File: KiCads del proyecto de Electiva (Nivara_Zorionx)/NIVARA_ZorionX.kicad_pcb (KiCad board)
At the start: 4 copper layers, 109.1 x 87.7 mm, 77 parts, among them J1 Screw_Terminal_01x03, J10 Screw_Terminal_01x03, J11 Screw_Terminal_01x03, J2 Screw_Terminal_01x03, J3 Screw_Terminal_01x04, J4 Screw_Terminal_01x03, J5 Screw_Terminal_01x02, J6 Screw_Terminal_01x02, J7 Screw_Terminal_01x03, J8 Screw_Terminal_01x04, J9 Screw_Terminal_01x06, K1 G2RL-1, K2 G2RL-1, U1 ESP32-S3-WROOM-1, U11 LTV-357TB, U12 LTV-357TB, U2 AP63200WU, U4 LTV-357TB, U5 LTV-357TB, U8 LTV-357TB, U9 LTV-357TB

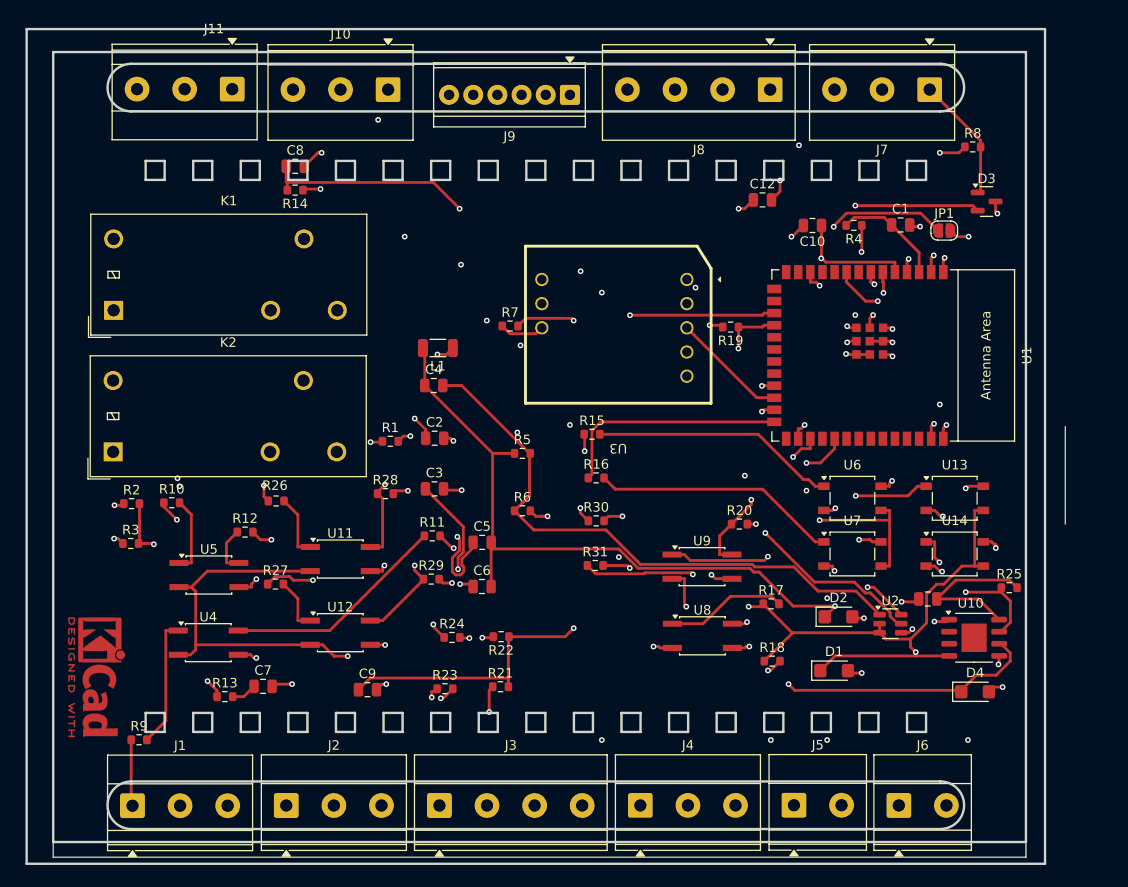
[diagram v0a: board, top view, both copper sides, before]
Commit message: Papadio Dame Fuerza
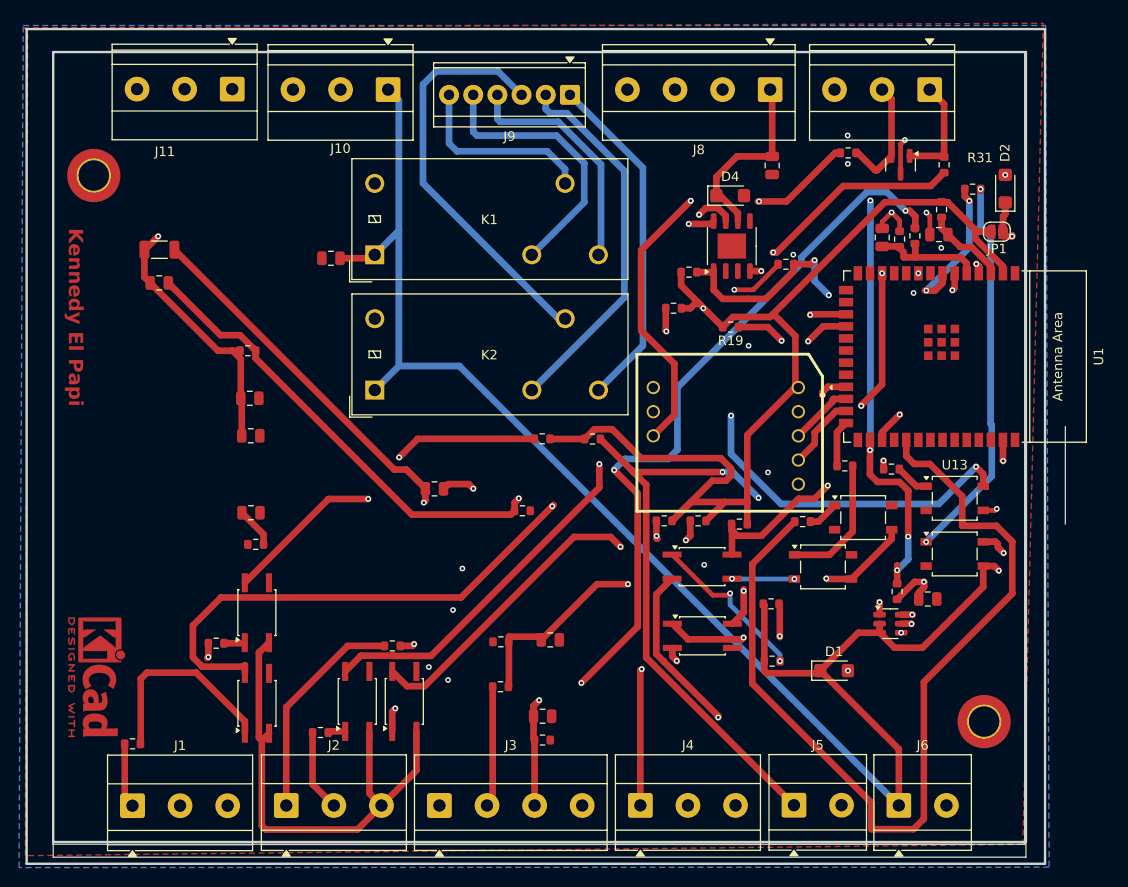
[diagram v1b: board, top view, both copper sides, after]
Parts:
- added REF**: MountingHole_3.2mm_M3_DIN965_Pad_TopOnly, MountingHole:MountingHole_3.2mm_M3_DIN965_Pad_TopOnly, F.Cu at (36.2, 41.4)
- added REF**: MountingHole_3.2mm_M3_DIN965_Pad_TopOnly, MountingHole:MountingHole_3.2mm_M3_DIN965_Pad_TopOnly, F.Cu at (129.7, 98.8)
- moved R3 74.8 mm to (108.9, 50.7)
- moved R23 68.6 mm to (122.5, 47.7), turned to -90 degrees
- moved R2 63.4 mm to (98.7, 51.5)
- moved C8 63.4 mm to (83.3, 98.2)
- moved R14 63.4 mm to (83.3, 100.7)
- moved R24 63.0 mm to (120.8, 48.1), turned to 90 degrees
- moved D4 58.1 mm to (103.0, 43.5)
- moved R31 56.0 mm to (128.5, 42.8)
- moved D2 48.3 mm to (131.9, 42.8), turned to 90 degrees
- moved U10 47.1 mm to (100.1, 49.2), turned to 90 degrees
- moved R7 39.9 mm to (115.4, 39.0)
- moved R29 38.2 mm to (97.1, 55.3)
- moved R28 33.0 mm to (99.7, 77.7)
- moved R12 32.7 mm to (83.3, 69.0)
- moved R30 31.5 mm to (120.0, 72.2)
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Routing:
- net +3.3V: track 20.2 -> 126.8 mm, vias 12 -> 2
- net GPIO16: track 134.2 -> 31.6 mm
- net GPIO5: track 102.5 -> 12.5 mm, vias 4 -> 0
- net /NIVARA_BOARD/+10V_AINPUT: track 13.0 -> 98.4 mm, vias 1 -> 3
- net /NIVARA_BOARD/VOLTAGE_AOUTPUT: track 93.1 -> 19.7 mm, vias 2 -> 0
- net GPIO38: track 30.3 -> 96.7 mm, vias 2 -> 0
- net /NIVARA_BOARD/RS485_B: track 74.6 -> 12.5 mm, vias 3 -> 0
- net GPIO1: track 134.1 -> 78.7 mm, vias 3 -> 2
- net GND: track 112.0 -> 62.7 mm, vias 46 -> 16
- net GPIO7: track 63.1 -> 16.0 mm, vias 3 -> 2
- net Net-(U10-V5V): track 17.0 -> 62.1 mm, vias 0 -> 3
- net /NIVARA_BOARD/Entradas_NPN/NPN_Output0: track 23.7 -> 67.5 mm, vias 0 -> 2
- net Net-(U3-B): track 4.75 -> 47.2 mm, vias 0 -> 2
- net GPIO6: track 57.1 -> 23.7 mm, vias 3 -> 2
- net /NIVARA_BOARD/Entradas_NPN/NPN_Output1: track 5.01 -> 37.3 mm, vias 0 -> 2
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- added copper zone on B.Cu, net GND
- added copper zone on F.Cu, net GND
- removed copper zone on In2.Cu, net GND
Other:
- outline, holes or cut-outs redrawn
- board text added: "Kennedy El Papi"
- board text added: "Pichardo lo más duro del Sistema"
